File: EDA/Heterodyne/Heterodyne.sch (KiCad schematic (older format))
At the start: 43 parts, among them J1 Conn_01x06, J7 Reciever, U1 SA612AD, U2 OPA2830, U3 MAX7375AXR105, U4 MAX11613, U5 ATmega328PB-AU, Y1 8 MHz

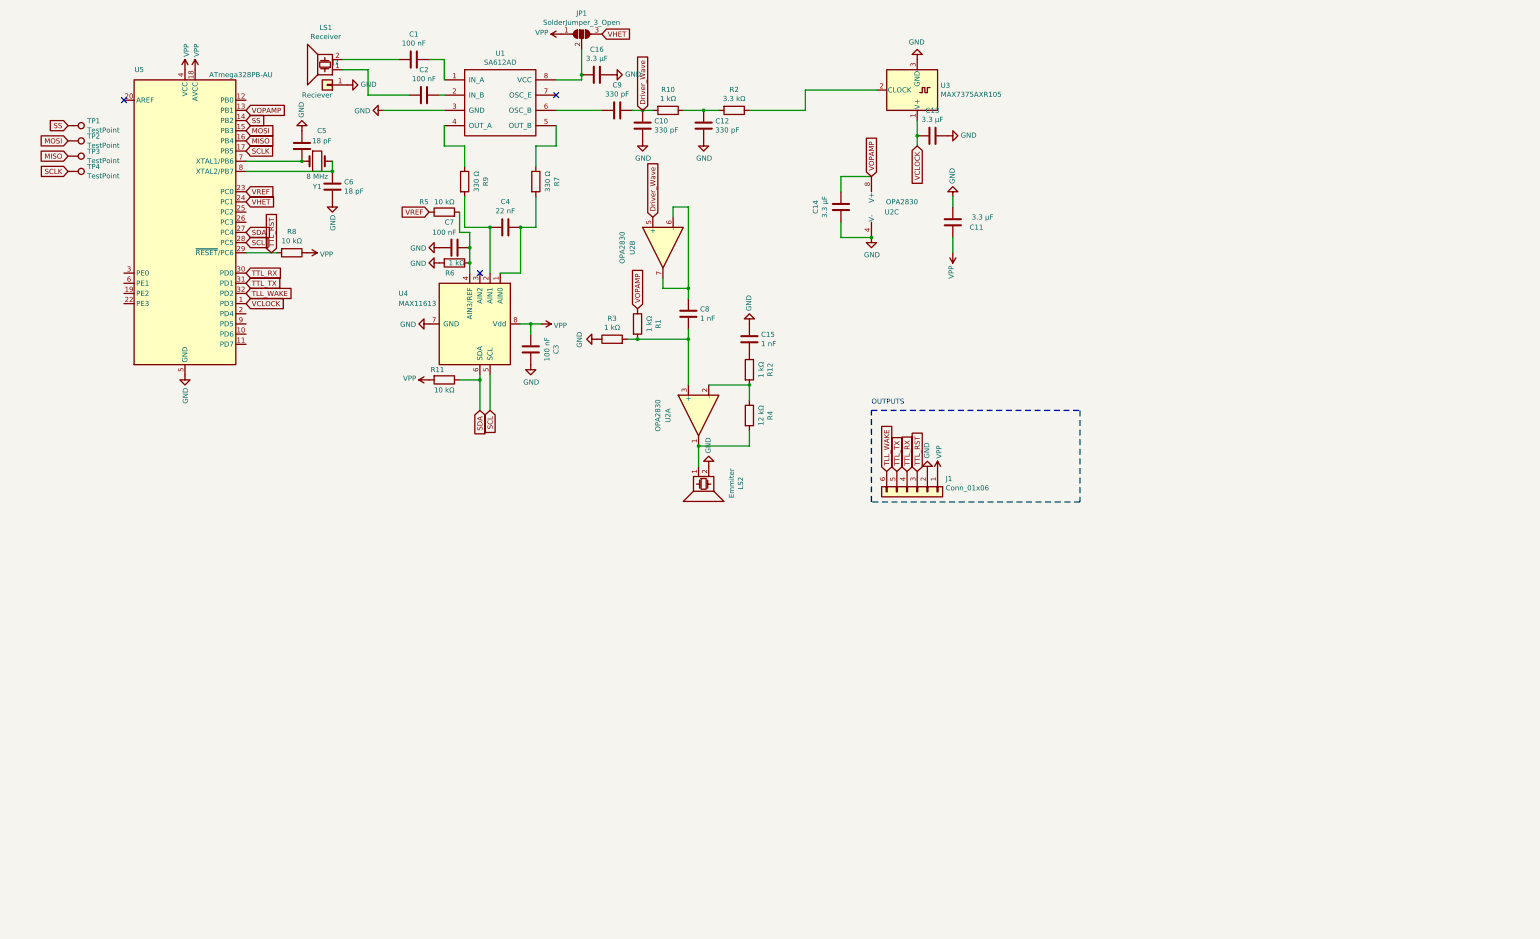
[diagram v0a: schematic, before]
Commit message: initial commit of SAMD21 branch
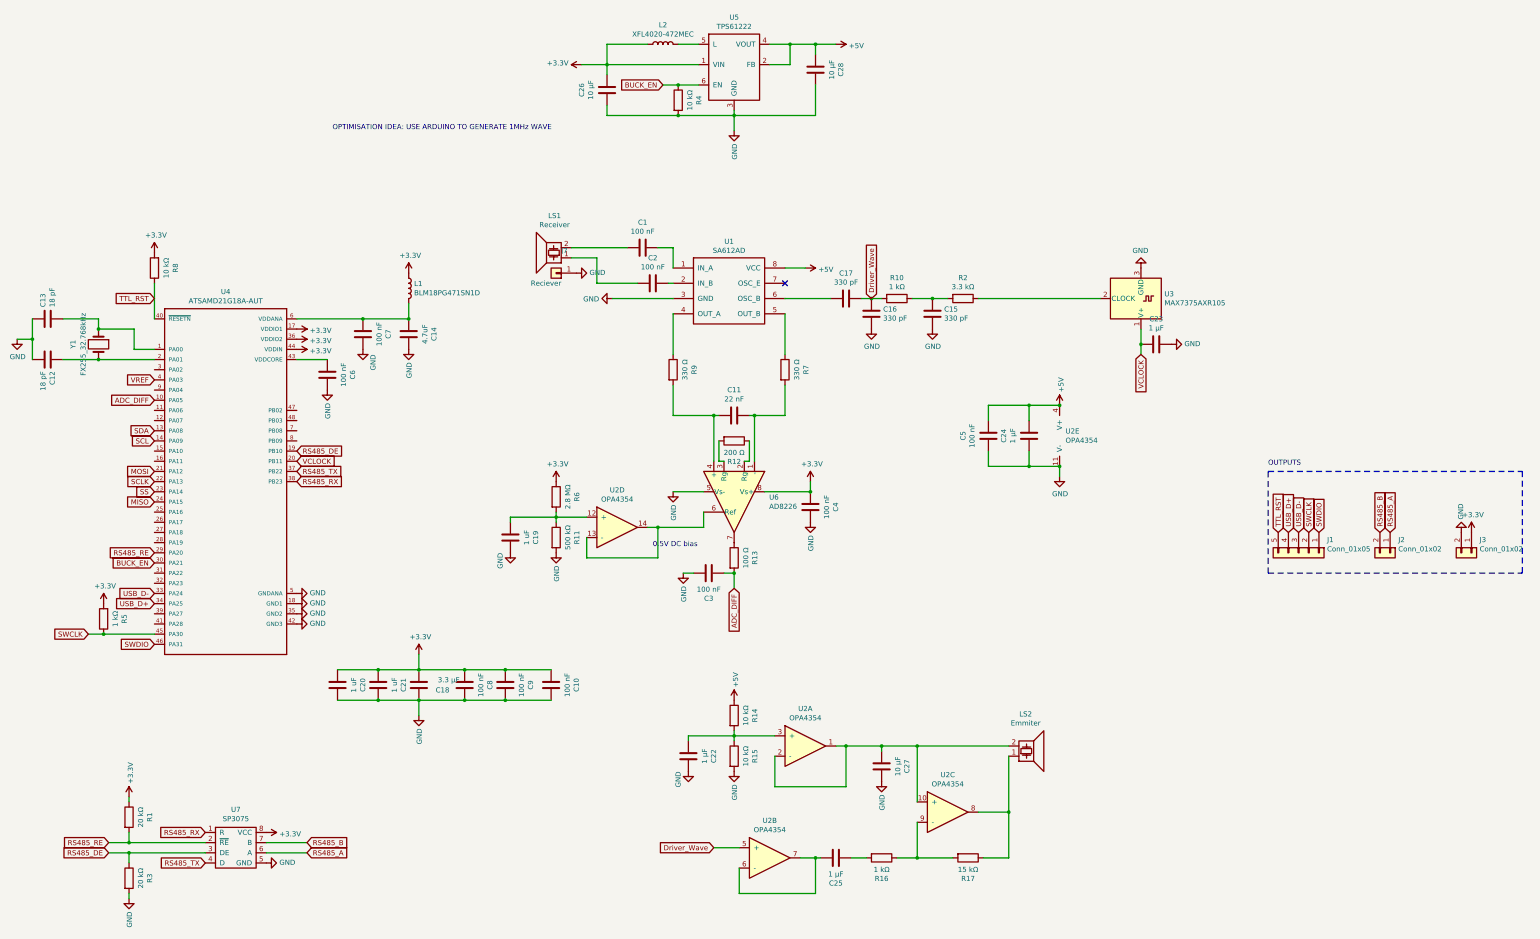
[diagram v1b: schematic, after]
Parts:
- removed C15, C8: 1 nF, Capacitor_SMD:C_0603_1608Metric, symbol Device:C
- removed C16: 3.3 μF, Capacitor_SMD:C_0805_2012Metric, symbol Heterodyne-rescue:C-Device
- removed C5, C6: 18 pF, Capacitor_SMD:C_0603_1608Metric, symbol Device:C
- removed J1: Conn_01x06, Connector_PinHeader_2.54mm:PinHeader_1x06_P2.54mm_Vertical, symbol Connector_Generic:Conn_01x06
- removed JP1: SolderJumper_3_Open, Jumper:SolderJumper-3_P1.3mm_Open_RoundedPad1.0x1.5mm_NumberLabels, symbol Jumper:SolderJumper_3_Open
- removed R11, R5: 10 kΩ, Resistor_SMD:R_0603_1608Metric, symbol Device:R
- removed R6: 1 kΩ, Resistor_SMD:R_0603_1608Metric, symbol Device:R
- removed TP1, TP2, TP3, TP4: TestPoint, Heterodyne:Testpoint SPI, symbol Connector:TestPoint
- removed U2: OPA2830, Package_SO:SOIC-8_3.9x4.9mm_P1.27mm, symbol Heterodyne-rescue:NE5532-Amplifier_Operational
- removed U4: MAX11613, Package_SO:MSOP-8_3x3mm_P0.65mm, symbol Analog_ADC:MAX11613
- removed U5: ATmega328PB-AU, Package_QFP:TQFP-32_7x7mm_P0.8mm, symbol MCU_Microchip_ATmega:ATmega328PB-AU
- added C10, C6, C8, C9: 100 nF, Capacitor_SMD:C_0402_1005Metric, symbol Heterodyne-rescue:C-Device
- added C12, C13: 18 pF, Capacitor_SMD:C_0603_1608Metric_Pad1.05x0.95mm_HandSolder, symbol Device:C
- added C14: 4.7uF, Capacitor_SMD:C_0603_1608Metric, symbol Heterodyne-rescue:C-Device
- added C19, C20, C21: 1 uF, Capacitor_SMD:C_0603_1608Metric_Pad1.05x0.95mm_HandSolder, symbol Heterodyne-rescue:C-Device
- added C22: 1 μF, Capacitor_SMD:C_0603_1608Metric_Pad1.05x0.95mm_HandSolder, symbol Heterodyne-rescue:C-Device
- added C25: 1 μF, Capacitor_SMD:C_0603_1608Metric, symbol Heterodyne-rescue:C-Device
- added C26, C27, C28: 10 μF, Capacitor_SMD:C_0805_2012Metric, symbol Heterodyne-rescue:C-Device
- added C4, C5: 100 nF, Capacitor_SMD:C_0603_1608Metric_Pad1.05x0.95mm_HandSolder, symbol Heterodyne-rescue:C-Device
- added J1: Conn_01x05, Connector_PinHeader_2.54mm:PinHeader_1x05_P2.54mm_Vertical, symbol Connector_Generic:Conn_01x05
- added J2, J3: Conn_01x02, Connector_PinHeader_2.54mm:PinHeader_1x02_P2.54mm_Vertical, symbol Connector_Generic:Conn_01x02
- added L1: BLM18PG471SN1D, Capacitor_SMD:C_0603_1608Metric, symbol Device:L
- added L2: XFL4020-472MEC, Inductor_SMD:L_Coilcraft_XxL4020, symbol Device:L
- added R11: 500 kΩ, Resistor_SMD:R_0603_1608Metric_Pad1.05x0.95mm_HandSolder, symbol Heterodyne-rescue:R-Device
- added R13: 100 Ω, Resistor_SMD:R_0603_1608Metric_Pad1.05x0.95mm_HandSolder, symbol Heterodyne-rescue:R-Device
- added R14, R15: 10 kΩ, Resistor_SMD:R_0603_1608Metric_Pad1.05x0.95mm_HandSolder, symbol Heterodyne-rescue:R-Device
- added R16: 1 kΩ, Resistor_SMD:R_0603_1608Metric_Pad1.05x0.95mm_HandSolder, symbol Heterodyne-rescue:R-Device
- added R17: 15 kΩ, Resistor_SMD:R_0603_1608Metric_Pad1.05x0.95mm_HandSolder, symbol Heterodyne-rescue:R-Device
- added R5: 1 kΩ, Resistor_SMD:R_0603_1608Metric, symbol Heterodyne-rescue:R-Device
- added R6: 2.8 MΩ, Resistor_SMD:R_0603_1608Metric_Pad1.05x0.95mm_HandSolder, symbol Heterodyne-rescue:R-Device
- added U2: OPA4354, symbol Amplifier_Operational:OPA4354
- added U4: ATSAMD21G18A-AUT, ATSAMD21G18A-AUT:QFP50P900X900X120-48N, symbol Heterodyne-rescue:ATSAMD21G18A-AUT-ATSAMD21G18A-AUT
- added U5: TPS61222, Package_TO_SOT_SMD:SOT-363_SC-70-6, symbol Regulator_Switching:TPS61222
- added U6: AD8226, Package_SO:SOIC-8_3.9x4.9mm_P1.27mm, symbol Amplifier_Instrumentation:AD8236
- added U7: SP3075, Package_SO:SOIC-8_3.9x4.9mm_P1.27mm, symbol Interface_UART:SN75176
- C1, C2, C3: footprint Capacitor_SMD:C_0603_1608Metric -> Capacitor_SMD:C_0603_1608Metric_Pad1.05x0.95mm_HandSolder
- C11: renamed from C4; footprint Capacitor_SMD:C_0603_1608Metric -> Capacitor_SMD:C_0603_1608Metric_Pad1.05x0.95mm_HandSolder
- C15: renamed from C12; footprint Capacitor_SMD:C_0603_1608Metric -> Capacitor_SMD:C_0603_1608Metric_Pad1.05x0.95mm_HandSolder
- C16: renamed from C10; footprint Capacitor_SMD:C_0603_1608Metric -> Capacitor_SMD:C_0603_1608Metric_Pad1.05x0.95mm_HandSolder
- C17: renamed from C9; footprint Capacitor_SMD:C_0603_1608Metric -> Capacitor_SMD:C_0603_1608Metric_Pad1.05x0.95mm_HandSolder
- C23: renamed from C13; value 3.3 μF -> 1 μF; footprint Capacitor_SMD:C_0805_2012Metric -> Capacitor_SMD:C_0603_1608Metric
- C24: renamed from C14; value 3.3 μF -> 1 μF; footprint Capacitor_SMD:C_0805_2012Metric -> Capacitor_SMD:C_0603_1608Metric
- C7: footprint Capacitor_SMD:C_0603_1608Metric -> Capacitor_SMD:C_0402_1005Metric
- R1, R3: value 1 kΩ -> 20 kΩ; footprint Resistor_SMD:R_0603_1608Metric -> Resistor_SMD:R_0603_1608Metric_Pad1.05x0.95mm_HandSolder
- R10, R2, R7, R8, R9: footprint Resistor_SMD:R_0603_1608Metric -> Resistor_SMD:R_0603_1608Metric_Pad1.05x0.95mm_HandSolder
- R12: value 1 kΩ -> 200 Ω; footprint Resistor_SMD:R_0603_1608Metric -> Resistor_SMD:R_0603_1608Metric_Pad1.05x0.95mm_HandSolder
- R4: value 12 kΩ -> 10 kΩ; footprint Resistor_SMD:R_0603_1608Metric -> Resistor_SMD:R_0603_1608Metric_Pad1.05x0.95mm_HandSolder
- Y1: value 8 MHz -> FX255_32.768kHz; footprint Crystal:Crystal_SMD_5032-2Pin_5.0x3.2mm -> Crystal:Crystal_SMD_MicroCrystal_CC4V-T1A-2Pin_5.0x1.9mm
- renumbered C11 to C18
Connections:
- net Driver_Wave: now also U2.5 (+)
- net GND: now also C18.1, C7.1, R3.2, R4.2, C10.1, C12.2, C13.1, C14.1, C19.1, C20.1, C21.1, C22.1, C26.2, C27.1, C28.1, C4.1, C5.2, C6.1, C8.1, C9.1, J3.2 (Pin_2), R11.2, R15.2, U2.11 (V-), U4.18 (GND1), U4.35 (GND2), U4.42 (GND3), U4.5 (GNDANA), U5.3 (GND), U6.5 (Vs-), U7.5 (GND); no longer C18.2, C7.2, LS2.2, R3.1
- net MISO: now also U4.24 (PA15)
- net MOSI: now also U4.21 (PA12)
- net SCL: now also U4.14 (PA09)
- net SCLK: now also U4.22 (PA13)
- net SDA: now also U4.13 (PA08)
- net SS: now also U4.23 (PA14)
- net TTL_RST: now also R8.1, J1.5 (Pin_5), U4.40 (~RESETN~); no longer R8.2
- net VCLOCK: now also U4.20 (PB11)
- net VREF: now also U4.4 (PA03)
- net +5V: now reaches U1.8 (VCC)
- net +5V: now also C24.1, C28.2, C5.1, R14.1, U2.4 (V+), U5.2 (FB), U5.4 (VOUT)
- net at LS2.1: now also R17.1, U2.8; no longer R4.2
- net at R12.2: now also U6.3 (Rg); no longer R4.1
- net RS485_RE: now reaches R1.2
- net RS485_RE: now also U4.29 (PA20), U7.2 (~RE); no longer R3.2
- net at C11.1, R7.2: now also U6.1 (-)
- net at C11.2, R9.2: now also U6.4 (+)
- net at Y1.1: now also C13.2, U4.1 (PA00)
- net at Y1.2: now also C12.1, U4.2 (PA01)
- net at R12.1: now also U6.2 (Rg)
- net VOPAMP renamed +3V3
- net +3V3: now also C18.2, R8.2, C10.2, C20.2, C21.2, C26.1, C4.2, C8.2, C9.2, J3.1 (Pin_1), L1.1, L2.1, R5.2, R6.1, U4.17 (VDDIO1), U4.36 (VDDIO2), U4.44 (VDDIN), U5.1 (VIN), U6.8 (Vs+), U7.8 (VCC); no longer C24.1
- removed net VPP: C18.1, C3.2, R8.1
- new net: C27.2, LS2.2, U2.1, U2.10 (+), U2.2 (-)
- new net: C6.2, U4.43 (VDDCORE)
- new net: C14.2, C7.2, L1.2, U4.6 (VDDANA)
- new net: U2.13 (-), U2.14, U6.6 (Ref)
- new net: R13.1, U6.7
- new net: C19.2, R11.1, R6.2, U2.12 (+)
- new net: C22.2, R14.2, R15.1, U2.3 (+)
- new net: C25.1, U2.6 (-), U2.7
- new net: C25.2, R16.2
- new net: R16.1, R17.2, U2.9 (-)
- new net: L2.2, U5.5 (L)
- new net ADC_DIFF: C3.2, R13.2, U4.10 (PA05)
- new net BUCK_EN: R4.1, U4.30 (PA21), U5.6 (EN)
- new net RS485_A: J2.1 (Pin_1), U7.6 (A)
- new net RS485_B: J2.2 (Pin_2), U7.7 (B)
- new net RS485_DE: R3.1, U4.19 (PB10), U7.3 (DE)
- new net RS485_RX: U4.38 (PB23), U7.1 (R)
- new net RS485_TX: U4.37 (PB22), U7.4 (D)
- new net SWCLK: J1.2 (Pin_2), R5.1, U4.45 (PA30)
- new net SWDIO: J1.1 (Pin_1), U4.46 (PA31)
- new net USB_D+: J1.4 (Pin_4), U4.34 (PA25)
- new net USB_D-: J1.3 (Pin_3), U4.33 (PA24)
- no-connect marks 3 -> 1
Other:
- note added: "0.5V DC bias"
- note added: "OPTIMISATION IDEA: USE ARDUINO TO GENERATE 1MHz WAVE"
- moved on the sheet: C1, C11, C15, C16, C17, C18, C2, C23, C24, J7, LS1, LS2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
